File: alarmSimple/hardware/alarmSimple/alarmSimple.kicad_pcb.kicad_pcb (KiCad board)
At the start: 2 copper layers, 72 x 53.2 mm, 38 parts, among them J1 Batt, J2 Conn_01x04_Male, Q1 AO3402_N_Mosfet, U1 chargeBoostBoard, U2 AMS1117-5.0

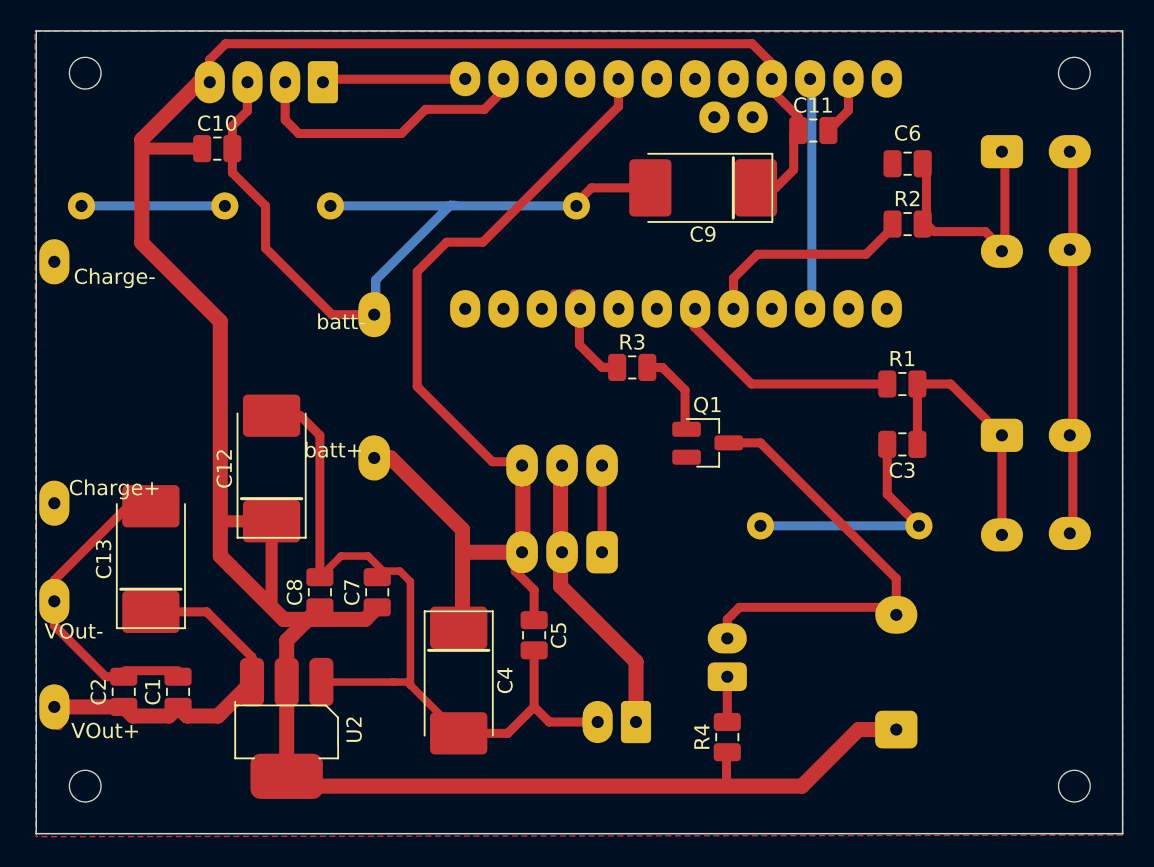
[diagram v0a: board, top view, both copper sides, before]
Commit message: finish arduino simple alarm design
finish arduino simple alarm design
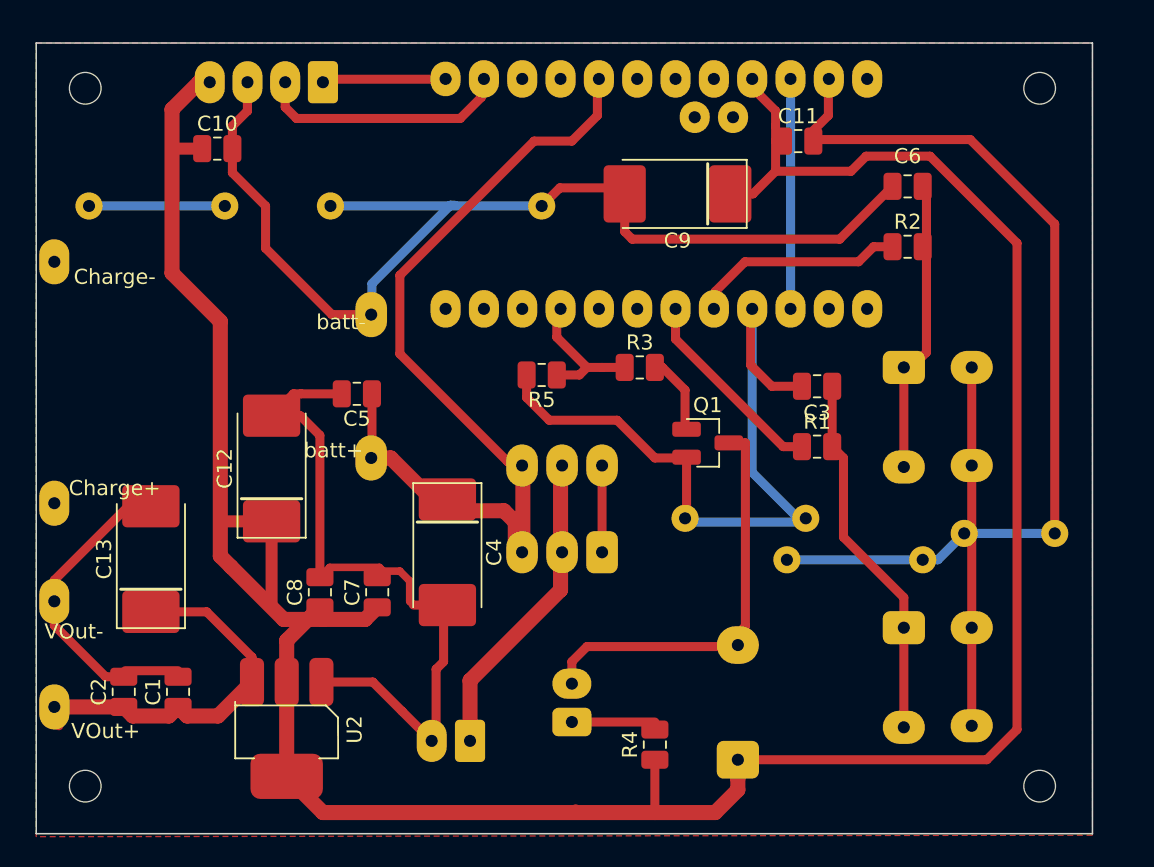
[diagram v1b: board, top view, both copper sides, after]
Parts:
- added R5: 10kR, myFootPrintLibs:R_C_0805_2012Metric_Pad_HandSolder, F.Cu at (62.0, 86.8)
- added REF**: via, myFootPrintLibs:via, F.Cu at (78.2, 99.0)
- added REF**: via, myFootPrintLibs:via, F.Cu at (79.5, 96.2)
- added REF**: via, myFootPrintLibs:via, F.Cu at (96.0, 97.2)
- added REF**: via, myFootPrintLibs:via, F.Cu at (90.0, 97.2)
- moved C5 19.9 mm to (49.8, 88.0), turned to 180 degrees
- moved S3 18.3 mm to (88.2, 89.8)
- moved S1 16.8 mm to (88.2, 107.0)
- moved J1 11.1 mm to (57.2, 111.0)
- moved D1 10.7 mm to (64.0, 109.8)
- moved BZ1 10.7 mm to (75.0, 112.2)
- moved C4 8.53 mm to (55.8, 98.5)
- moved R1 7.01 mm to (80.2, 91.5)
- moved C3 6.84 mm to (80.2, 87.5)
- moved REF** 5.02 mm to (71.5, 96.2)
- moved R4 4.83 mm to (69.5, 111.2)
- moved   2.51 mm to (95.0, 67.8)
- moved ? 2.30 mm to (95.0, 114.0)
- moved REF** 2.30 mm to (62.0, 75.5)
- moved REF** 2.26 mm to (87.2, 99.0)
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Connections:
- net /Out5.8V renamed Net-(C1-Pad1)
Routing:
- net GND: track 183.9 -> 286.5 mm
- net +5V: track 171.5 -> 192.1 mm
- net Net-(C3-Pad1): track 17.6 -> 24.7 mm
- net VBattCheck: track 65.8 -> 60.0 mm
- net Net-(C6-Pad1): track 16.5 -> 19.7 mm
- net buzz_en: track 6.92 -> 9.87 mm
- net button_plus: track 16.2 -> 13.3 mm
- net Net-(BZ1-Pad2): track 29.8 -> 27.2 mm
- net Net-(B1-Pad11): track 19.3 -> 16.8 mm
- net Net-(D1-PadA): track 3.40 -> 5.50 mm
- net Net-(J1-Pad1): track 19.3 -> 21.0 mm
- net Net-(B1-Pad10): track 9.48 -> 8.22 mm
- net button_minus: track 13.3 -> 14.0 mm
- net Net-(B1-PadRST): track 15.7 -> 15.1 mm
- net Net-(Q1-PadG): track 5.76 -> 5.26 mm
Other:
- board size 72 x 53.2 mm -> 70 x 52.4 mm
